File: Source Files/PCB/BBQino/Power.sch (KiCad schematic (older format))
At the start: 29 parts, among them IC1 VOD205T, J1 VIN < 13V, J4 Screw_Terminal_01x02, Q1 IPD068P03L3G, Q2 DMP4051LK3, Q3 DMN4040SK3, Q4 DMP4051LK3, Q5 DMN4040SK3, U1 ADP7142ARDZ-5.0, U2 INA219AxD

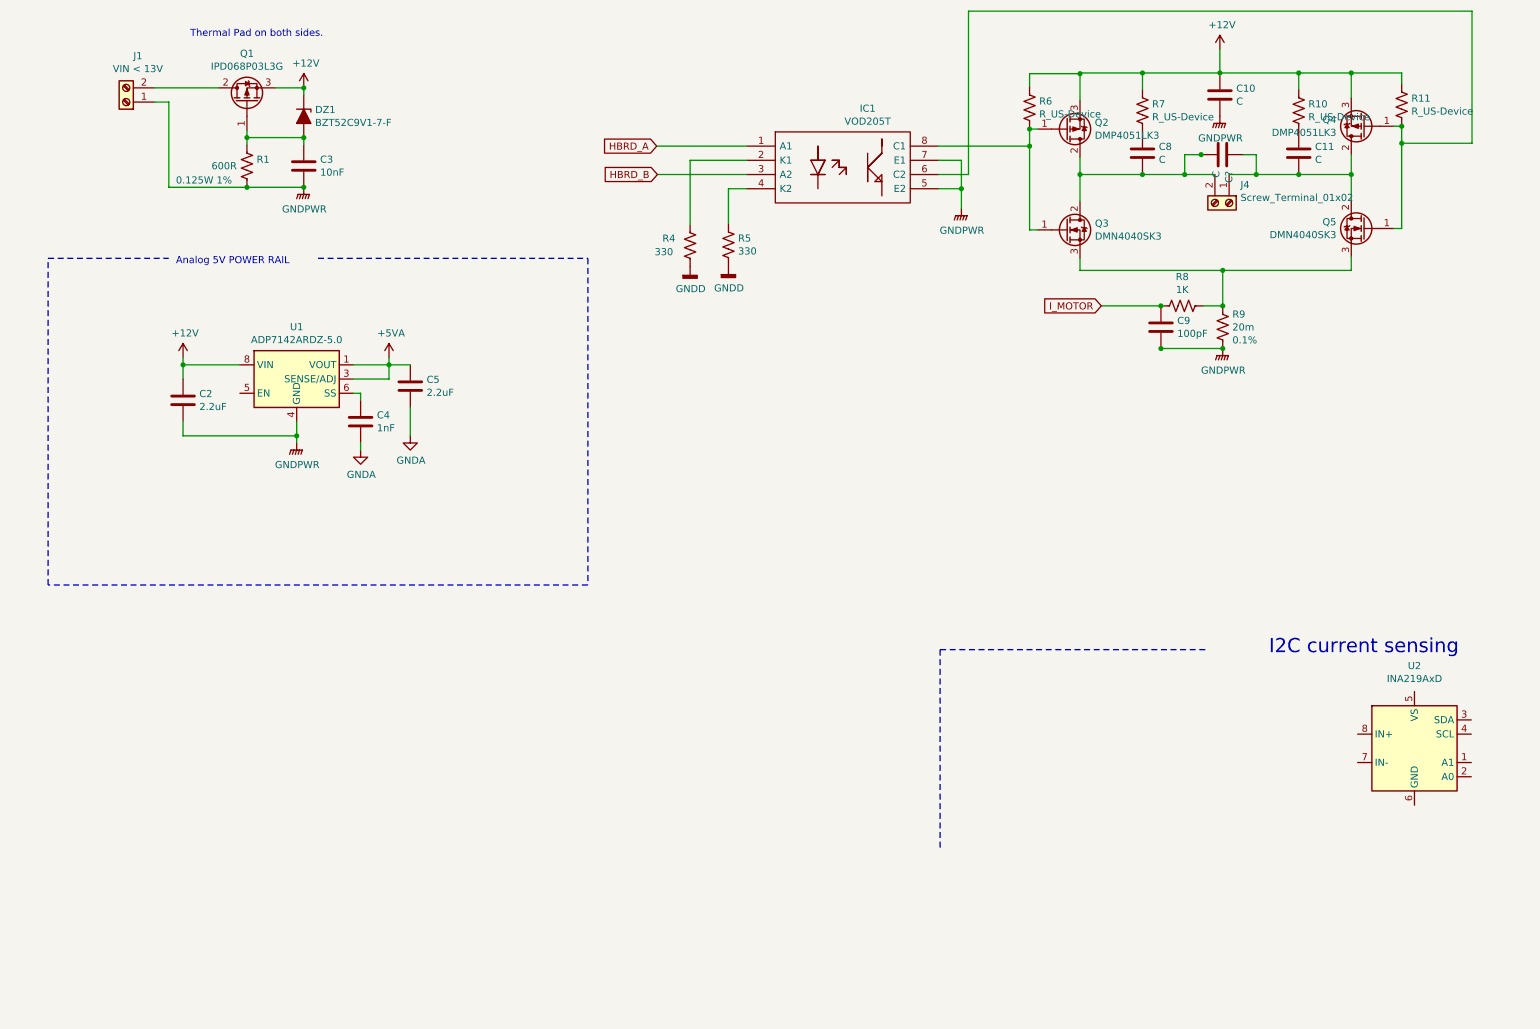
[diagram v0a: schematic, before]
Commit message: New architecture
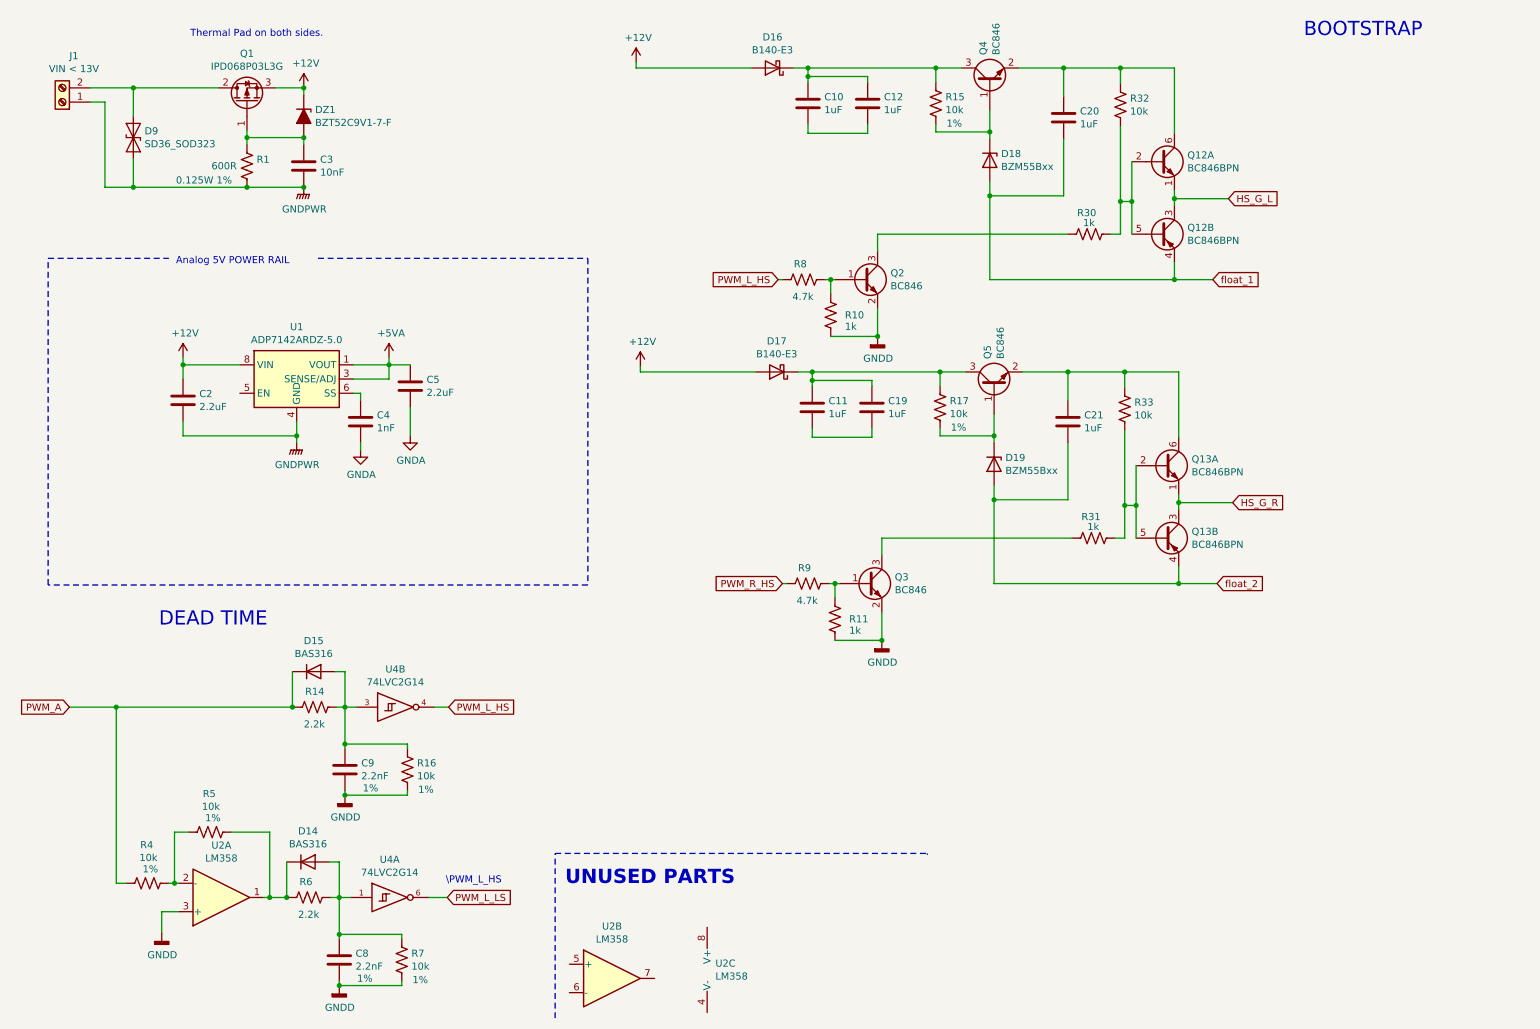
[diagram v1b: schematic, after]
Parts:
- removed C10, C11, C8, C?: C, symbol Device:C
- removed C9: 100pF, symbol Device:C
- removed IC1: VOD205T, SOIC127P610X323-8N, symbol BBQino-rescue:VOD205T
- removed J4: Screw_Terminal_01x02, symbol Connector:Screw_Terminal_01x02
- removed Q2, Q4: DMP4051LK3, Package_TO_SOT_SMD:TO-252-3_TabPin2, symbol Device:Q_PMOS_GDS
- removed Q3, Q5: DMN4040SK3, Package_TO_SOT_SMD:TO-252-3_TabPin2, symbol Device:Q_NMOS_GDS
- removed U2: INA219AxD, Package_SO:SOIC-8_3.9x4.9mm_P1.27mm, symbol Analog_ADC:INA219AxD
- added C10, C11, C12, C19, C20, C21: 1uF, Capacitor_SMD:C_0805_2012Metric_Pad1.18x1.45mm_HandSolder, symbol BBQino-rescue:C-Device
- added C8, C9: 2.2nF, Capacitor_SMD:C_0805_2012Metric_Pad1.18x1.45mm_HandSolder, symbol BBQino-rescue:C-Device
- added D14, D15: BAS316, Diode_SMD:D_SOD-323, symbol Diode:BAS316
- added D16, D17: B140-E3, Diode_SMD:D_SMA, symbol Diode:B140-E3
- added D18, D19: BZM55Bxx, Diode_SMD:D_MicroMELF, symbol Diode:BZM55Bxx
- added D9: SD36_SOD323, Diode_SMD:D_SOD-323, symbol Diode:SD36_SOD323
- added Q12, Q13: BC846BPN, Package_TO_SOT_SMD:SOT-363_SC-70-6, symbol Transistor_BJT:BC846BPN
- added Q2, Q3, Q4, Q5: BC846, Package_TO_SOT_SMD:SOT-23, symbol Transistor_BJT:BC846
- added R14: 2.2k, symbol BBQino-rescue:R_US-Device
- added R15, R16, R17, R32, R33: 10k, symbol BBQino-rescue:R_US-Device
- added R30, R31: 1k, symbol BBQino-rescue:R_US-Device
- added U2: LM358, symbol Amplifier_Operational:LM358
- added U4: 74LVC2G14, symbol 74xGxx:74LVC2G14
- R10, R11: value R_US-Device -> 1k
- R4, R5: value 330 -> 10k; footprint Resistor_SMD:R_0805_2012Metric_Pad1.20x1.40mm_HandSolder -> (none); Value2 (none) -> 1%
- R6: value R_US-Device -> 2.2k; Value2 (none) -> 1%
- R7: value R_US-Device -> 10k; Value2 (none) -> 1%
- R8: value 1K -> 4.7k
- R9: value 20m -> 4.7k; Value2 0.1% -> (none)
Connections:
- net labels added: HS_G_L, HS_G_R, PWM_A, PWM_L_HS, PWM_L_LS, PWM_R_HS, float_1, float_2
- net labels removed: HBRD_A, HBRD_B, I_MOTOR
- wire segments 90 -> 167
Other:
- note added: "BOOTSTRAP\n"
- note added: "DEAD TIME\n"
- note added: "UNUSED PARTS"
- note added: "\PWM_L_HS\n"
- note removed: "I2C current sensing\n"
- moved on the sheet: J1
